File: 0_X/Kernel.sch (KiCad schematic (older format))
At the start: 14 parts, among them J1 TTL, J2 L, J3 R, J4 TTL, SW1 MODE, SW2 Reset, SW3 RePair, U1 ESP-12S

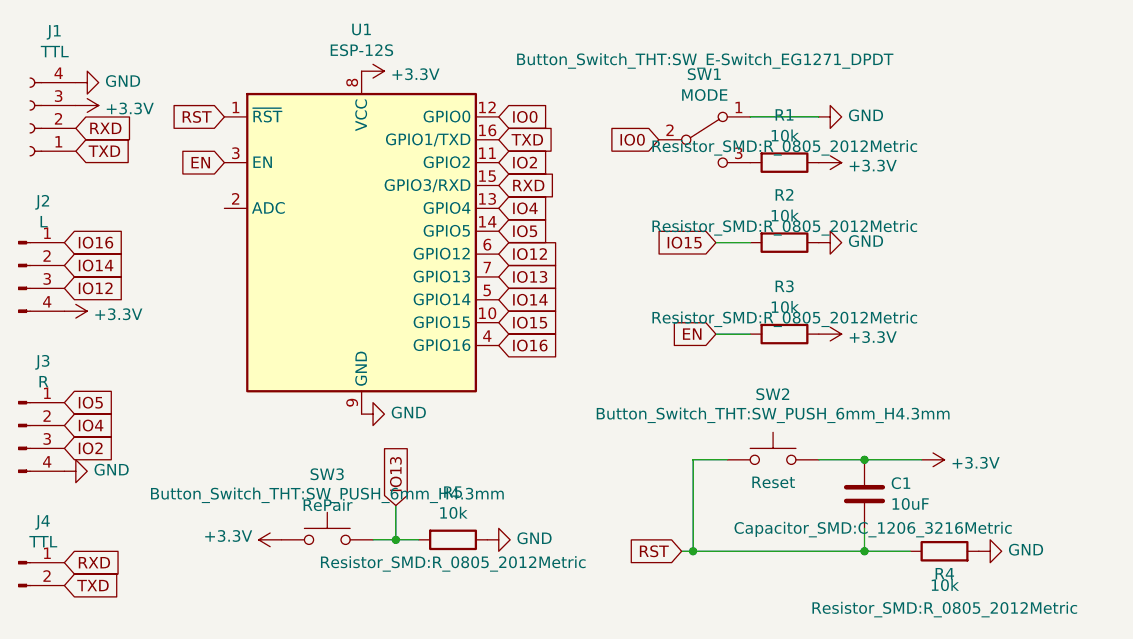
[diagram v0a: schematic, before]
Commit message: update Ver 1.1
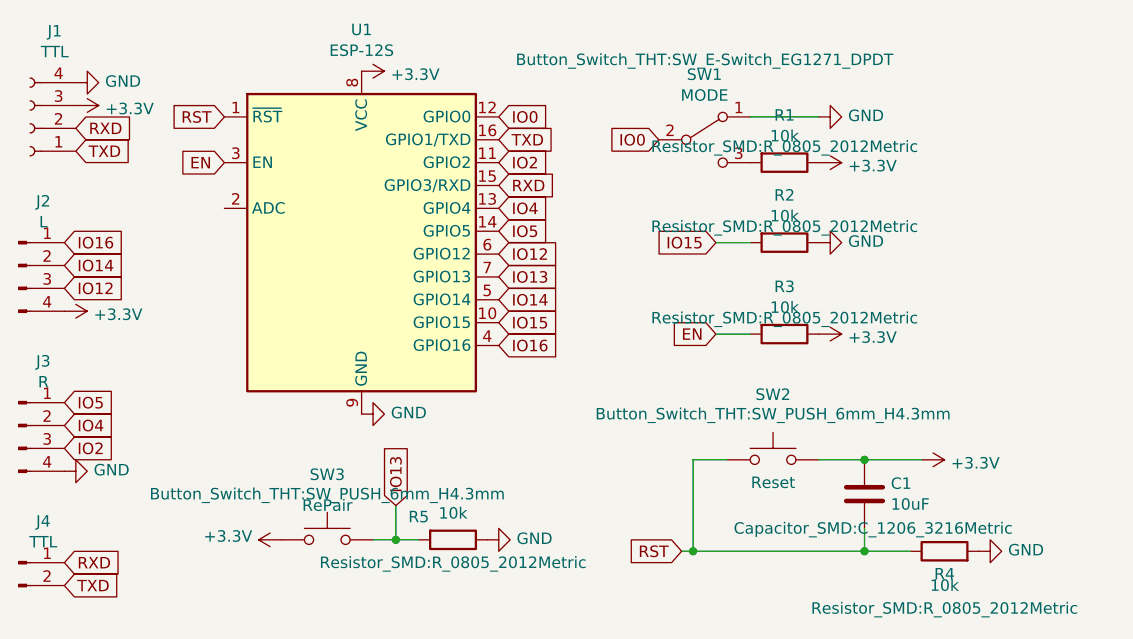
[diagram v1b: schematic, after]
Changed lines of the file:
@@
 $EndComp
-$Comp
-L Connector:Conn_01x04_Female J1
-U 1 1 6049A723
-P 4000 3200
-F 0 "J1" H 3892 2775 50  0000 C CNN
-F 1 "TTL" H 3892 2866 50  0000 C CNN
-F 2 "Connector_PinHeader_2.54mm:PinHeader_1x04_P2.54mm_Horizontal" H 4000 3200 50  0001 C CNN
-F 3 "~" H 4000 3200 50  0001 C CNN
-	1    4000 3200
-	-1   0    0    1
-$EndComp
-$Comp
-L power:GND #PWR0110
-U 1 1 6049DE5E
-P 4200 3000
-F 0 "#PWR0110" H 4200 2750 50  0001 C CNN
-F 1 "GND" V 4205 2872 50  0000 R CNN
-F 2 "" H 4200 3000 50  0001 C CNN
-F 3 "" H 4200 3000 50  0001 C CNN
-	1    4200 3000
-	0    -1   -1   0
-$EndComp
-Text GLabel 4200 3300 2    50   Input ~ 0
-TXD
-Text GLabel 4200 3200 2    50   Input ~ 0
-RXD
 $Comp
 L Kernel-rescue:ESP-12S-RF_Module U1
@@
 U 1 1 604EF1A5
 P 5850 5000
-F 0 "R5" V 5643 5000 50  0000 C CNN
+F 0 "R5" V 5750 4850 50  0000 C CNN
 F 1 "10k" V 5734 5000 50  0000 C CNN
 F 2 "Resistor_SMD:R_0805_2012Metric" V 5950 5000 50  0000 C CNN
@@
 IO2
 $Comp
+L Switch:SW_SPDT SW1
+U 1 1 6048DEAF
+P 6950 3250
+F 0 "SW1" H 6950 3535 50  0000 C CNN
+F 1 "MODE" H 6950 3444 50  0000 C CNN
+F 2 "Button_Switch_THT:SW_E-Switch_EG1271_DPDT" H 6950 3600 50  0000 C CNN
+F 3 "~" H 6950 3250 50  0001 C CNN
+	1    6950 3250
+	1    0    0    -1
+$EndComp
+$Comp
+L Switch:SW_Push SW2
+U 1 1 604A6E52
+P 7250 4650
+F 0 "SW2" H 7250 4935 50  0000 C CNN
+F 1 "Reset" H 7250 4550 50  0000 C CNN
+F 2 "Button_Switch_THT:SW_PUSH_6mm_H4.3mm" H 7250 4850 50  0000 C CNN
+F 3 "~" H 7250 4850 50  0001 C CNN
+	1    7250 4650
+	1    0    0    -1
+$EndComp
+$Comp
+L Connector:Conn_01x02_Male J4
+U 1 1 60571445
+P 3950 5100
+F 0 "J4" H 4058 5281 50  0000 C CNN
+F 1 "TTL" H 4058 5190 50  0000 C CNN
+F 2 "Connector_PinHeader_2.54mm:PinHeader_1x02_P2.54mm_Vertical" H 3950 5100 50  0001 C CNN
+F 3 "~" H 3950 5100 50  0001 C CNN
+	1    3950 5100
+	1    0    0    -1
+$EndComp
+Text GLabel 4150 5200 2    50   Input ~ 0
+TXD
+Text GLabel 4150 5100 2    50   Input ~ 0
+RXD
+$Comp
+L Switch:SW_Push SW3
+U 1 1 604DDF37
+P 5300 5000
+F 0 "SW3" H 5300 5285 50  0000 C CNN
+F 1 "RePair" H 5300 5150 50  0000 C CNN
+F 2 "Button_Switch_THT:SW_PUSH_6mm_H4.3mm" H 5300 5200 50  0000 C CNN
+F 3 "~" H 5300 5200 50  0001 C CNN
+	1    5300 5000
+	1    0    0    -1
+$EndComp
+$Comp
 L power:+3.3V #PWR0109
 U 1 1 6049D3BD
@@
 	0    1    1    0
 $EndComp
-$Comp
-L Switch:SW_SPDT SW1
-U 1 1 6048DEAF
-P 6950 3250
-F 0 "SW1" H 6950 3535 50  0000 C CNN
-F 1 "MODE" H 6950 3444 50  0000 C CNN
-F 2 "Button_Switch_THT:SW_E-Switch_EG1271_DPDT" H 6950 3600 50  0000 C CNN
-F 3 "~" H 6950 3250 50  0001 C CNN
-	1    6950 3250
-	1    0    0    -1
-$EndComp
-$Comp
-L Switch:SW_Push SW2
-U 1 1 604A6E52
-P 7250 4650
-F 0 "SW2" H 7250 4935 50  0000 C CNN
-F 1 "Reset" H 7250 4550 50  0000 C CNN
-F 2 "Button_Switch_THT:SW_PUSH_6mm_H4.3mm" H 7250 4850 50  0000 C CNN
-F 3 "~" H 7250 4850 50  0001 C CNN
-	1    7250 4650
-	1    0    0    -1
-$EndComp
-$Comp
-L Connector:Conn_01x02_Male J4
-U 1 1 60571445
-P 3950 5100
-F 0 "J4" H 4058 5281 50  0000 C CNN
-F 1 "TTL" H 4058 5190 50  0000 C CNN
-F 2 "Connector_PinHeader_2.54mm:PinHeader_1x02_P2.54mm_Vertical" H 3950 5100 50  0001 C CNN
-F 3 "~" H 3950 5100 50  0001 C CNN
-	1    3950 5100
-	1    0    0    -1
-$EndComp
-Text GLabel 4150 5200 2    50   Input ~ 0
+Text GLabel 4200 3200 2    50   Input ~ 0
+RXD
+Text GLabel 4200 3300 2    50   Input ~ 0
 TXD
-Text GLabel 4150 5100 2    50   Input ~ 0
-RXD
-$Comp
-L Switch:SW_Push SW3
-U 1 1 604DDF37
-P 5300 5000
-F 0 "SW3" H 5300 5285 50  0000 C CNN
-F 1 "RePair" H 5300 5150 50  0000 C CNN
-F 2 "Button_Switch_THT:SW_PUSH_6mm_H4.3mm" H 5300 5200 50  0000 C CNN
-F 3 "~" H 5300 5200 50  0001 C CNN
-	1    5300 5000
-	1    0    0    -1
+$Comp
+L power:GND #PWR0110
+U 1 1 6049DE5E
+P 4200 3000
+F 0 "#PWR0110" H 4200 2750 50  0001 C CNN
+F 1 "GND" V 4205 2872 50  0000 R CNN
+F 2 "" H 4200 3000 50  0001 C CNN
+F 3 "" H 4200 3000 50  0001 C CNN
+	1    4200 3000
+	0    -1   -1   0
+$EndComp
+$Comp
+L Connector:Conn_01x04_Female J1
+U 1 1 6049A723
+P 4000 3200
+F 0 "J1" H 3892 2775 50  0000 C CNN
+F 1 "TTL" H 3892 2866 50  0000 C CNN
+F 2 "Connector_PinHeader_2.54mm:PinHeader_1x04_P2.54mm_Horizontal" H 4000 3200 50  0001 C CNN
+F 3 "~" H 4000 3200 50  0001 C CNN
+	1    4000 3200
+	-1   0    0    1
 $EndComp
 $EndSCHEMATC
